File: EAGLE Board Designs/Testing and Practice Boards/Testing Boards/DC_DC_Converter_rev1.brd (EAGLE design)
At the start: 99.9 x 58.7 mm, 17 parts, among them U1 DCM3714BD2K13E0C09

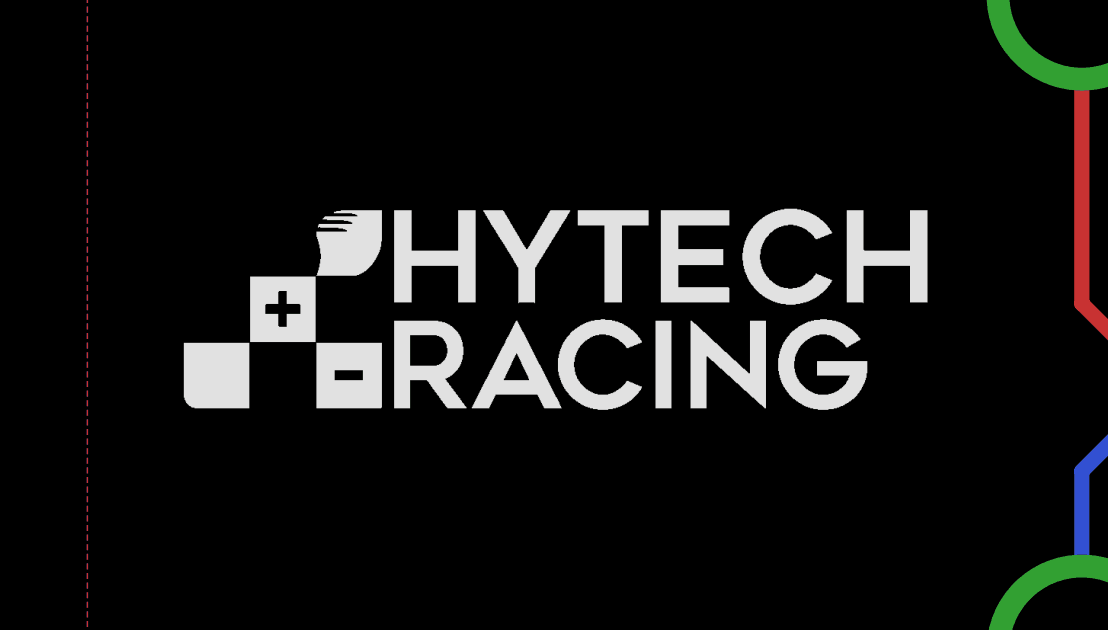
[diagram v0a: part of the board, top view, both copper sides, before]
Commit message: Final changes made
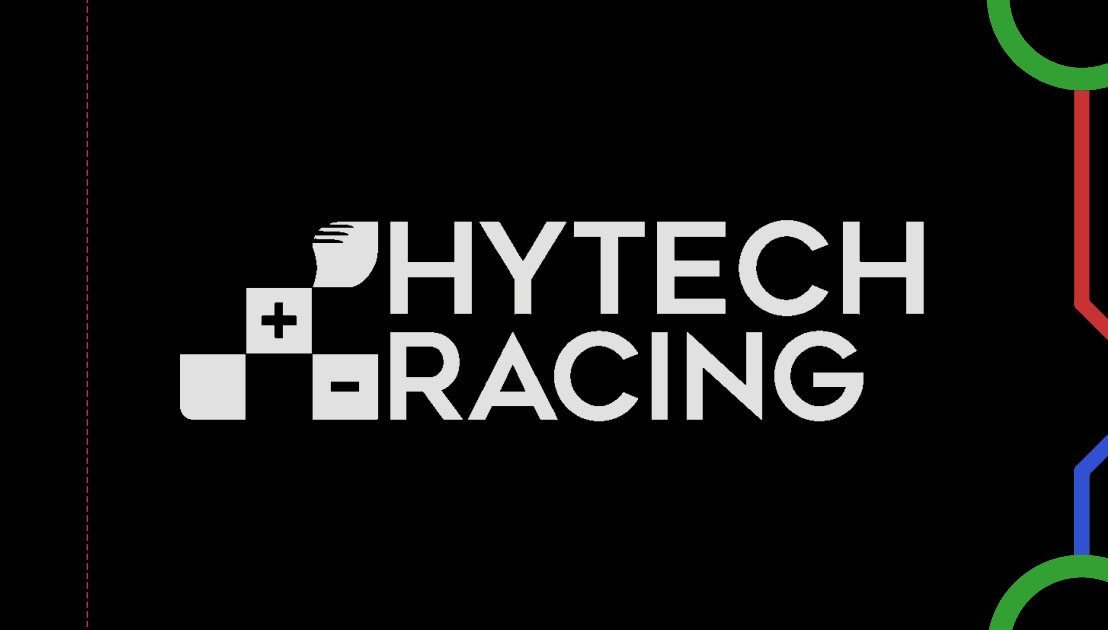
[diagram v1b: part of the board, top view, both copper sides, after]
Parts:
- moved U$6 0.40 mm to (63.4, 16.4)
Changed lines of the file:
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@@
 <element name="U$2" library="HyTechAesthetics" package="HV_0.50&quot;" value="" x="35.56" y="34.29" smashed="yes"/>
 <element name="U$3" library="HyTechAesthetics" package="HV_0.50&quot;" value="" x="48.26" y="52.07" smashed="yes"/>
-<element name="U$6" library="HyTechAesthetics" package="LOGO_HYTECH_1.0&quot;" value="" x="63.5" y="16.764" smashed="yes"/>
+<element name="U$6" library="HyTechAesthetics" package="LOGO_HYTECH_1.0&quot;" value="" x="63.373" y="16.383" smashed="yes"/>
 <element name="U$7" library="HyTechAesthetics" package="LOGO_GT_0.50&quot;" value="" x="49.53" y="20.32" smashed="yes"/>
 <element name="U$8" library="HyTechAesthetics" package="HV_0.50&quot;" value="" x="35.56" y="5.08" smashed="yes" rot="MR0"/>
